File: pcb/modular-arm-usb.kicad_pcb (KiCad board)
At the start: 2 copper layers, 8.7 x 12 mm, 28 parts, among them CON1 ARM-SWD-HEADER, IC1 LPC11U14FBD48, P1 USB, P2 UNFUSED_PWR, P3 BATT, P4 GPIO, P5 BATT, P6 GPIO2, U2 MCP1700T-3302E/TT, U3 nRF24L01+, X1 16M xtal

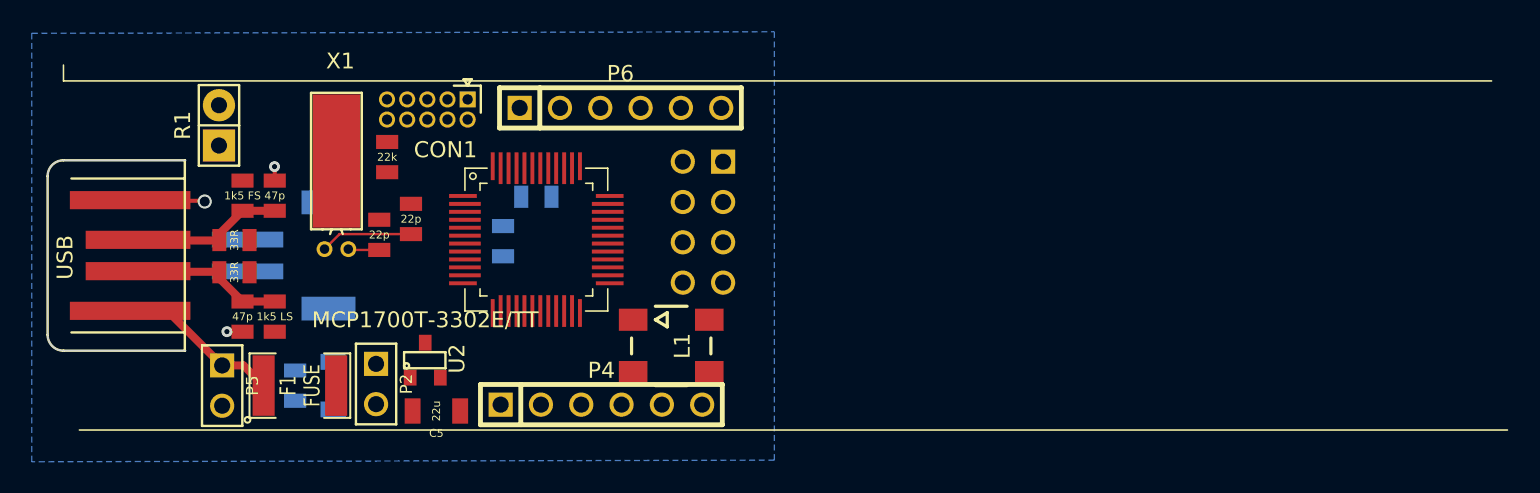
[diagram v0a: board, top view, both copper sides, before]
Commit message: pcb work from last night
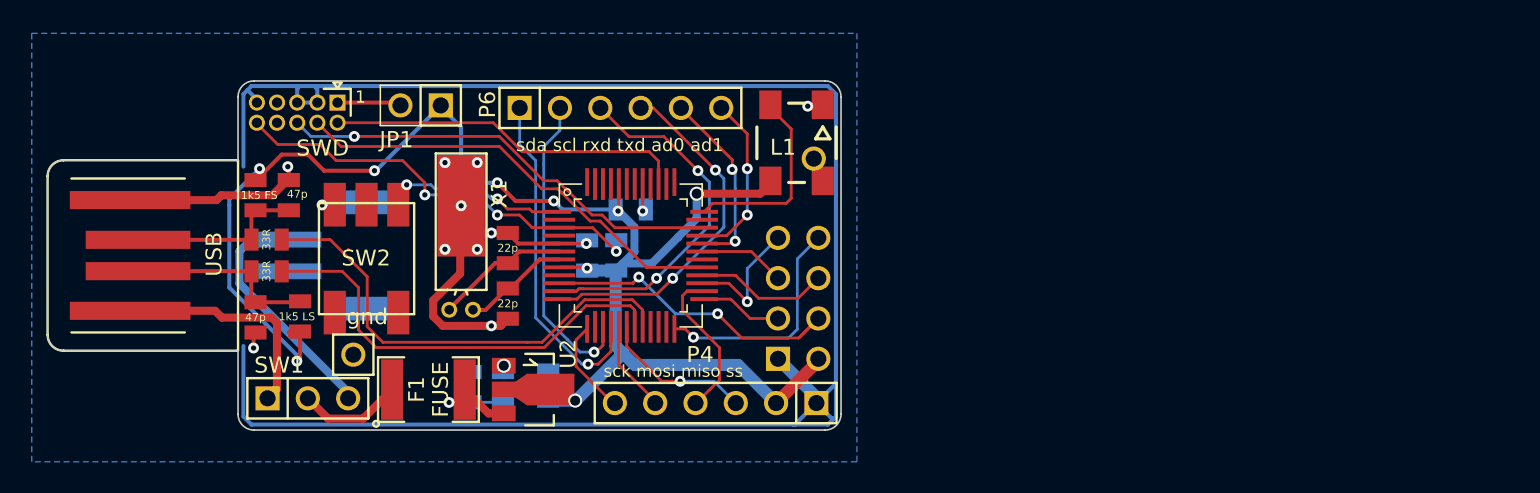
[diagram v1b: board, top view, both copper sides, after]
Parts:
- removed R1: NC, Pin_Headers:Pin_Header_Straight_1x02
- added JP1: NC, myelin:PIN_ARRAY_2X1, F.Cu at (96.2, 82.5)
- added SW1: SW_SPDT, myelin:PIN_ARRAY_3X1, F.Cu at (90.4, 101.0)
- added SW2: SW_PUSH_ALT, OMRON-PUSH-BUTTON-B3SN-3112P:OMRON-PUSH-BUTTON-B3SN-3112P, F.Cu at (94.1, 92.2)
- C1, C2, C6, C7, C8, C9, R3, R4, R5, R6: footprint SM0805_NOSILKSCREEN -> myelin:SM0805_NOSILKSCREEN
- C3: value 22u -> 10u; footprint myelin:SM1206_nosilkscreen -> myelin:SM0805_NOSILKSCREEN
- C5: value 22u -> 10u; footprint myelin:SM1206_nosilkscreen -> myelin:SM0805_NOSILKSCREEN; moved to B.Cu
- CON1: value ARM-SWD-HEADER -> SWD
- F1: footprint SM1812 -> SMD_Packages:SMD-1812
- IC1: footprint NXP_LQFP48_BY_HAND -> myelin:NXP_LQFP48_BY_HAND
- L1: footprint WS2812B_PP -> myelin:WS2812B_PP
- P1: footprint USB_A_PCB -> myelin:USB_A_PCB
- P2: value UNFUSED_PWR -> LED; footprint PIN_ARRAY_2X1 -> Pin_Headers:Pin_Header_Straight_1x01; moved to B.Cu
- P3: footprint S2B-PH-SM4-TB(LF)(SN) -> myelin:S2B-PH-SM4-TB(LF)(SN)
- P4, P6: footprint PIN_ARRAY-6X1 -> myelin:PIN_ARRAY_6X1
- P5: value BATT -> gnd; footprint PIN_ARRAY_2X1 -> Pin_Headers:Pin_Header_Straight_1x01
- R2: footprint SM0805_NOSILKSCREEN -> myelin:SM0805_NOSILKSCREEN; moved to B.Cu
- U2: value MCP1700T-3302E/TT -> MCP1700T; footprint SMD_Packages:SOT-23 -> Housings_SOT-89:SOT89-3_Housing
- U3: footprint NRF24L01_MODULE -> myelin:NRF24L01_MODULE
- moved P2 31.0 mm to (122.3, 85.9), turned to 0 degrees
- moved R2 15.7 mm to (109.8, 92.0)
- moved L1 15.0 mm to (121.2, 84.9), turned to 0 degrees
- moved C4 11.1 mm to (100.7, 100.3), turned to 90 degrees
- moved C3 10.7 mm to (102.7, 100.3), turned to 90 degrees
- moved C7 9.19 mm to (103.0, 95.0), turned to 90 degrees
- moved X1 8.74 mm to (100.1, 95.4)
- moved P5 8.49 mm to (93.3, 98.3), turned to 0 degrees
- moved CON1 8.20 mm to (91.0, 83.0)
- moved F1 8.10 mm to (98.0, 100.5)
- moved U3 7.68 mm to (121.3, 94.7), turned to 90 degrees
- moved C5 7.23 mm to (105.5, 100.2), turned to 90 degrees
- moved P4 7.20 mm to (116.1, 101.3), turned to 180 degrees
- moved U2 7.05 mm to (104.6, 100.5), turned to 270 degrees
- moved C6 6.37 mm to (103.0, 91.5)
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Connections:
- F1 pad 1: VUSB -> /power/VIN
- IC1 pad 1: Net-(IC1-Pad1) -> /lpc-mcu/BUTTON
- IC1 pad 23: /lpc-mcu/LED_INPUT -> Net-(IC1-Pad23)
- IC1 pad 36: Net-(IC1-Pad36) -> /lpc-mcu/LED_INPUT
- P2 pad 1: Net-(C3-Pad1) -> Net-(L1-Pad2)
- P3 pad 2: VUSB -> /power/VBATT
- P4 pad 3: /lpc-mcu/SCL -> /lpc-mcu/SSEL1
- P4 pad 4: /lpc-mcu/SDA -> /lpc-mcu/MISO1
- P4 pad 5: /lpc-mcu/RXD -> /lpc-mcu/MOSI1
- P4 pad 6: /lpc-mcu/TXD -> /lpc-mcu/SCK1
- P5 pad 1: VUSB -> GND
- P6 pad 1: /lpc-mcu/AD0 -> /lpc-mcu/SDA
- P6 pad 2: /lpc-mcu/AD1 -> /lpc-mcu/SCL
- P6 pad 3: /lpc-mcu/SSEL1 -> /lpc-mcu/RXD
- P6 pad 4: /lpc-mcu/MISO1 -> /lpc-mcu/TXD
- P6 pad 5: /lpc-mcu/MOSI1 -> /lpc-mcu/AD0
- P6 pad 6: /lpc-mcu/SCK1 -> /lpc-mcu/AD1
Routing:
- net GND: track 5.99 -> 171.6 mm, vias 3 -> 14
- net 3V3: track 0.00 -> 104.0 mm, vias 0 -> 9
- net LPC_USB_DP: track 0.00 -> 29.7 mm
- net /lpc-mcu/SWO: track 0.00 -> 28.5 mm, vias 0 -> 1
- net /lpc-mcu/SWCLK: track 0.00 -> 28.2 mm
- net LPC_USB_DM: track 0.00 -> 28.1 mm
- net /lpc-mcu/nRESET: track 0.00 -> 27.2 mm, vias 0 -> 3
- net /lpc-mcu/RXD: track 0.00 -> 23.6 mm, vias 0 -> 2
- net /lpc-mcu/SWDIO: track 0.00 -> 22.7 mm
- net /lpc-mcu/TXD: track 0.00 -> 22.5 mm, vias 0 -> 2
- net /lpc-mcu/SDA: track 0.00 -> 21.5 mm, vias 0 -> 1
- net RF24_CSN: track 0.00 -> 20.3 mm, vias 0 -> 2
- net /lpc-mcu/SCL: track 0.00 -> 19.5 mm, vias 0 -> 1
- net /power/VBATT: track 0.00 -> 15.3 mm
- net RF24_IRQ: track 0.00 -> 14.5 mm, vias 0 -> 1
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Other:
- board size 8.7 x 12 mm -> 50 x 22 mm
- board text added: "1"
- board text added: "3v3"
- board text added: "github.com/ myelin/ modular-arm-usb v1 phil pearson & phil lindsay"
- board text added: "sck mosi miso ss"
- board text added: "sda scl rxd txd ad0 ad1"
